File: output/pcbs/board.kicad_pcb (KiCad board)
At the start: 2 copper layers, 122.3 x 101.1 mm, 39 parts

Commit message: wip
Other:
- net class Power added: clearance 0.2, trace_width 0.5, via_dia 0.8, via_drill 0.4
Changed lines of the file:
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@@
 (net 39 "P8")
 (net 40 "P9")
-  (net_class Default "This is the default net class."
+  (net_class Default "This is the default net class"
     (clearance 0.2)
     (trace_width 0.25)
@@
 (add_net "home_thumb")
 (add_net "far_thumb")
-(add_net "RAW")
-(add_net "GND")
 (add_net "RST")
-(add_net "VCC")
 (add_net "P14")
 (add_net "P16")
@@
 (add_net "P9")
   )
+  (net_class Power "This is the power net class"
+    (clearance 0.2)
+    (trace_width 0.5)
+    (via_dia 0.8)
+    (via_drill 0.4)
+    (uvia_dia 0.3)
+    (uvia_drill 0.1)
+    (add_net "RAW")
+(add_net "GND")
+(add_net "VCC")
+  )
       (module PG1350 (layer F.Cu)

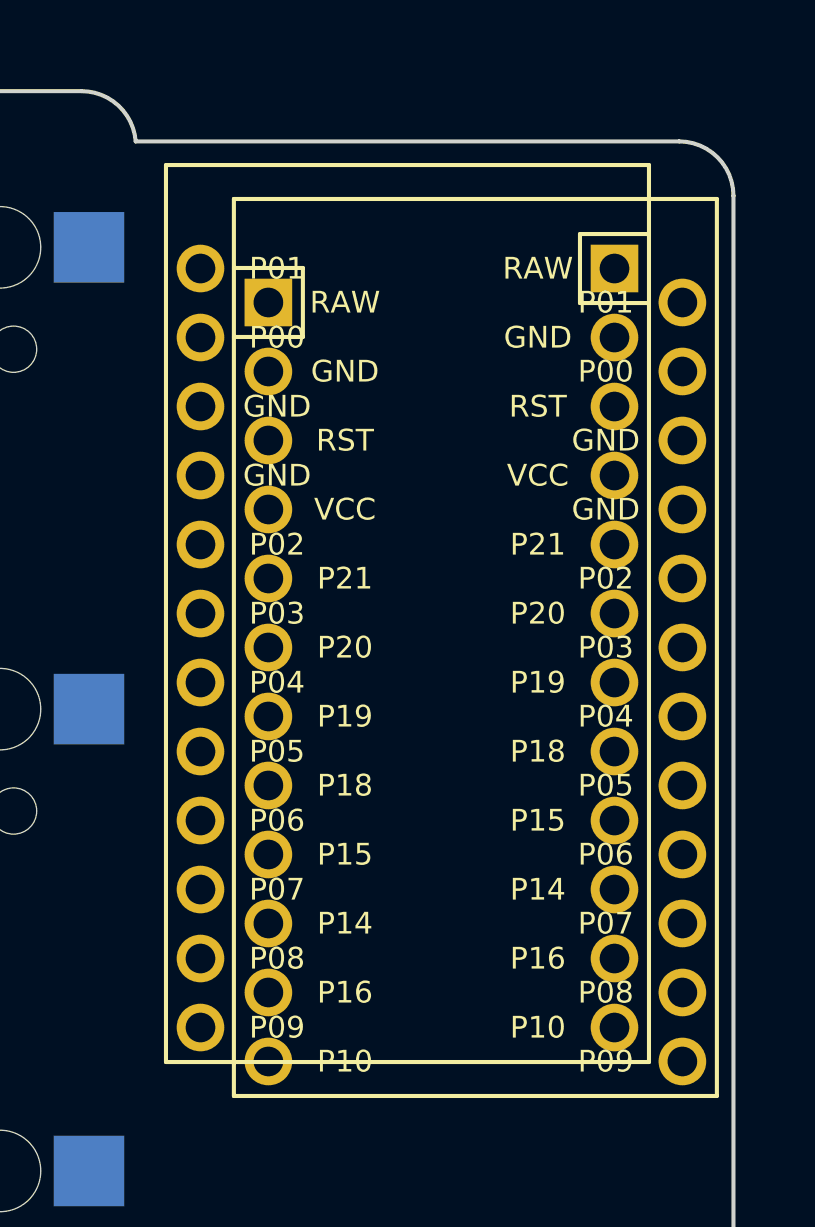
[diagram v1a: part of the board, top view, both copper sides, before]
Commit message: A probably working version
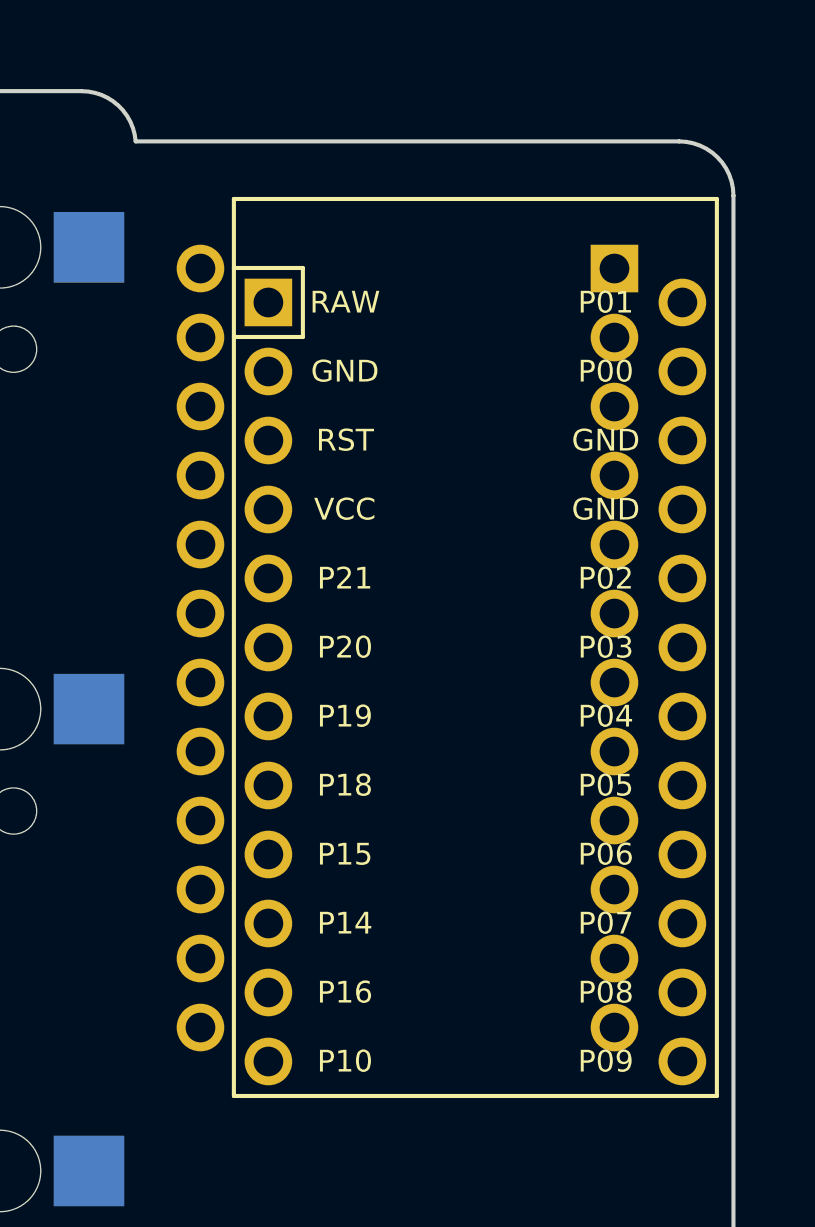
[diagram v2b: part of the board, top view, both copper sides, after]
